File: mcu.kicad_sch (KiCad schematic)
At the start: 14 parts, among them J10 M3, J11 Conn_01x10, J7 M0, J8 M1, J9 M2, SW1 Push_Button, SW2 Push_Button, U2 ESP32-S3-WROOM-1

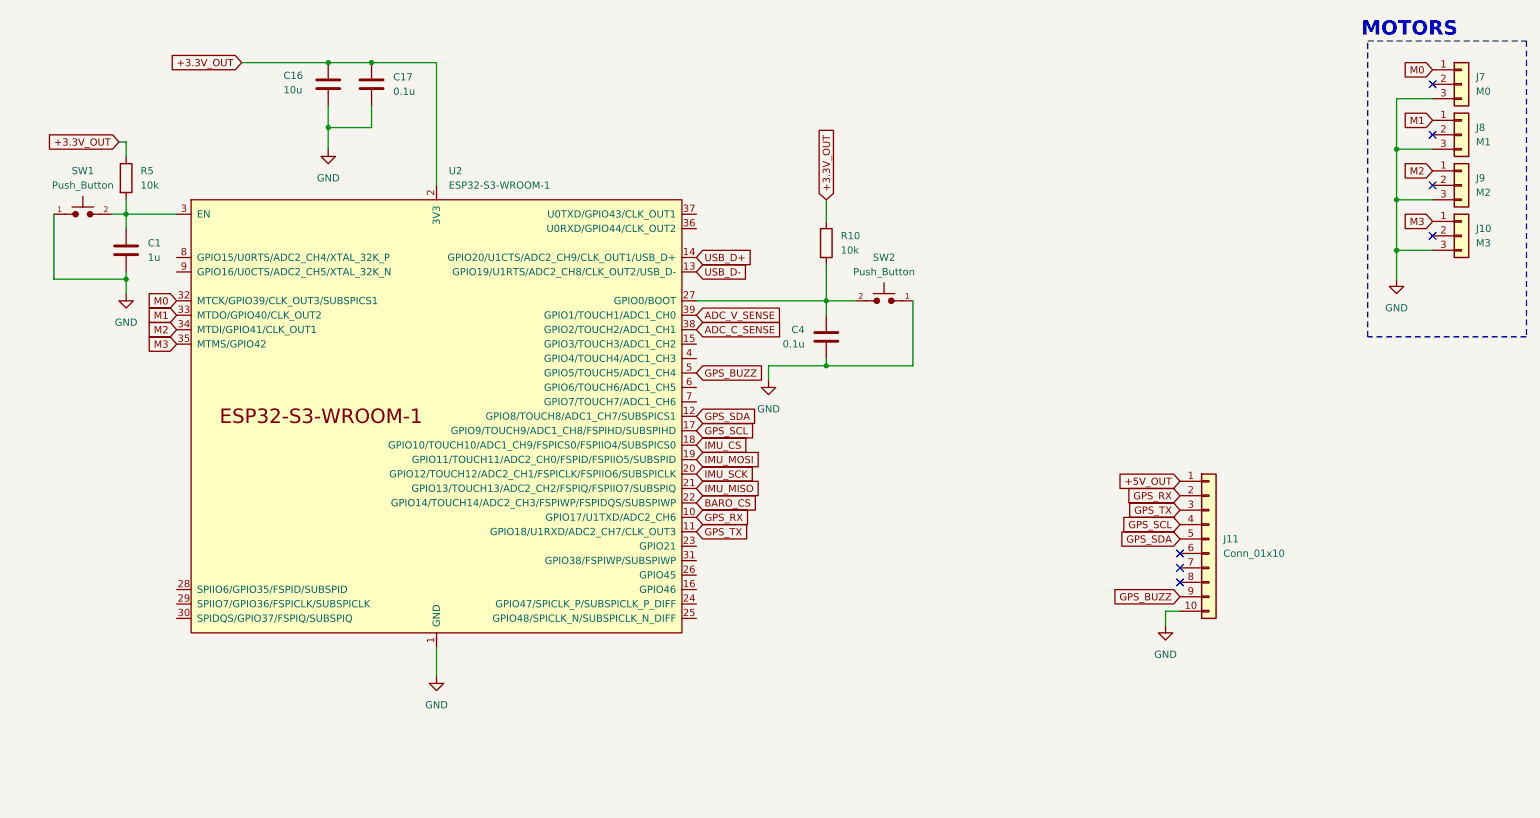
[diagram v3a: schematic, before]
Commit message: 8.09.2026 - 23:26
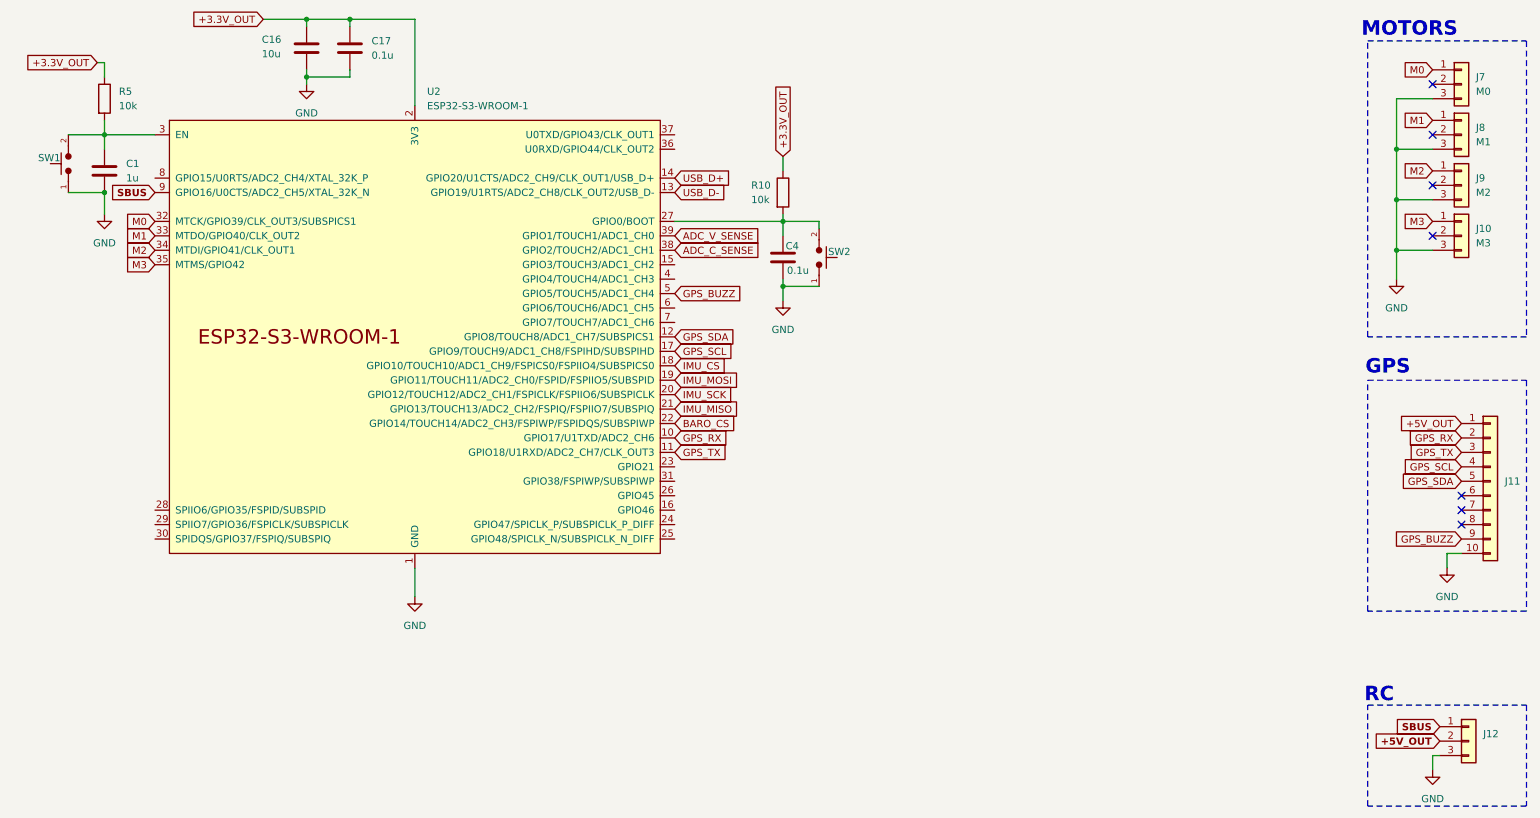
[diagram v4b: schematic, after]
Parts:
- added J12: Conn_01x03, symbol Connector_Generic:Conn_01x03
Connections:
- net +5V_OUT: now also J12.2 (Pin_2)
- net GND: now also J12.3 (Pin_3)
- net SBUS: now reaches U2.9 (GPIO16/U0CTS/ADC2_CH5/XTAL_32K_N)
- net SBUS: now also J12.1 (Pin_1)
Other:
- note added: "GPS"
- note added: "RC"
- moved on the sheet: C1, C16, C17, C4, J11, R10, R5, SW1, SW2, U2

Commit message: 9.09.2026 - 00:22
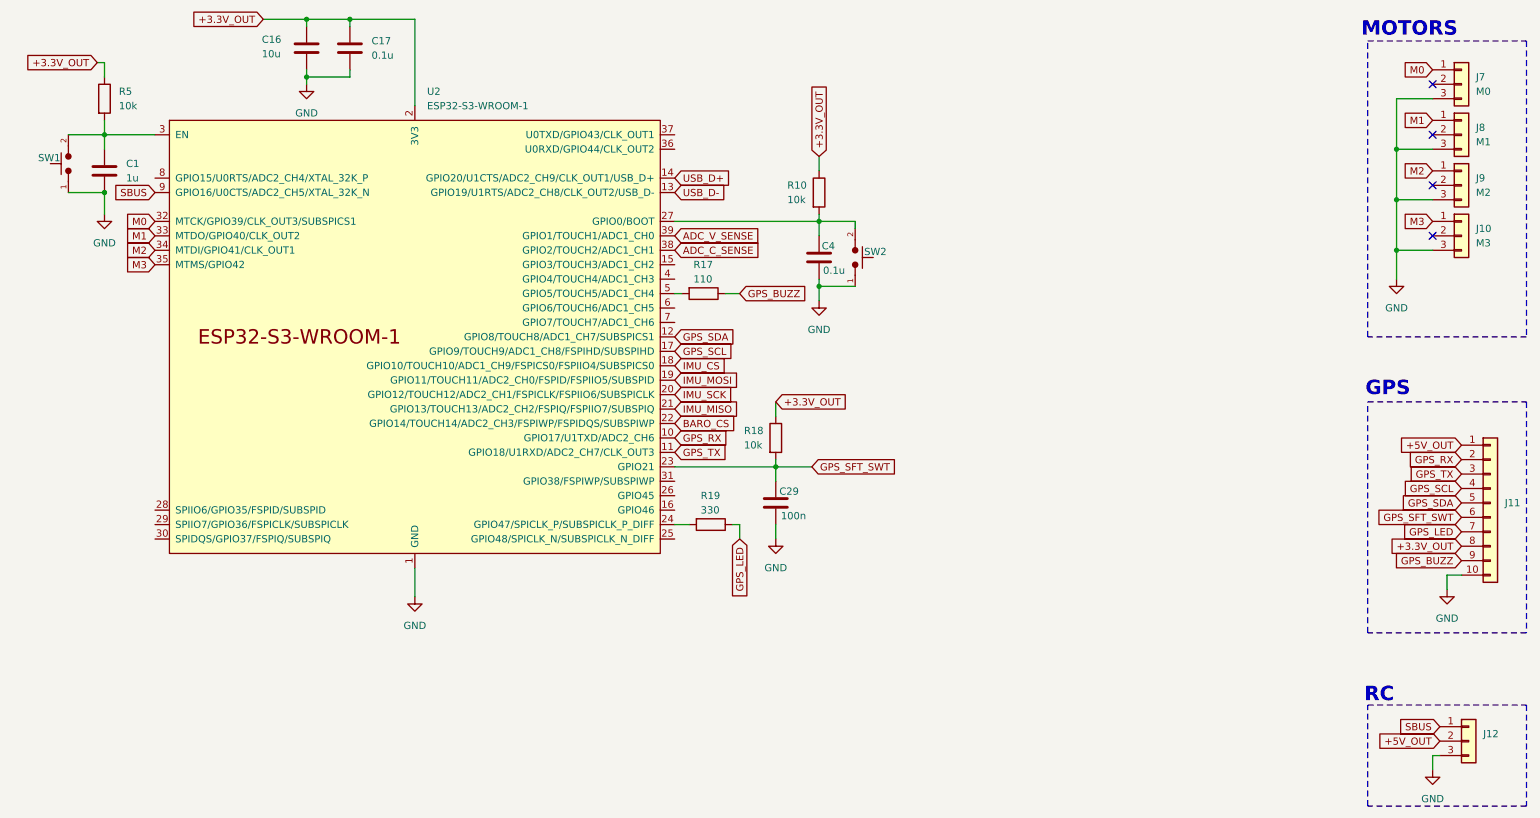
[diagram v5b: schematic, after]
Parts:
- added C29: 100n, symbol Device:C
- added R17: 110, symbol Device:R
- added R18: 10k, symbol Device:R
- added R19: 330, symbol Device:R
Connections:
- net +3.3V_OUT: now also J11.8 (Pin_8), R18.1
- net GND: now also C29.2
- net GPS_BUZZ: now also R17.1; no longer U2.5 (GPIO5/TOUCH5/ADC1_CH4)
- net GPS_SFT_SWT: now reaches U2.23 (GPIO21)
- net GPS_SFT_SWT: now also J11.6 (Pin_6), C29.1, R18.2
- net at U2.24 (GPIO47/SPICLK_P/SUBSPICLK_P_DIFF): now also R19.2
- net GPS_LED: now reaches J11.7 (Pin_7)
- net GPS_LED: now also R19.1
- new net: R17.2, U2.5 (GPIO5/TOUCH5/ADC1_CH4)
- no-connect marks 7 -> 4
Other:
- moved on the sheet: C4, J11, R10, SW2
